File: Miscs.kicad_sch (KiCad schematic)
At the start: 14 parts, among them U7 THGBMUG6C1LBAIL

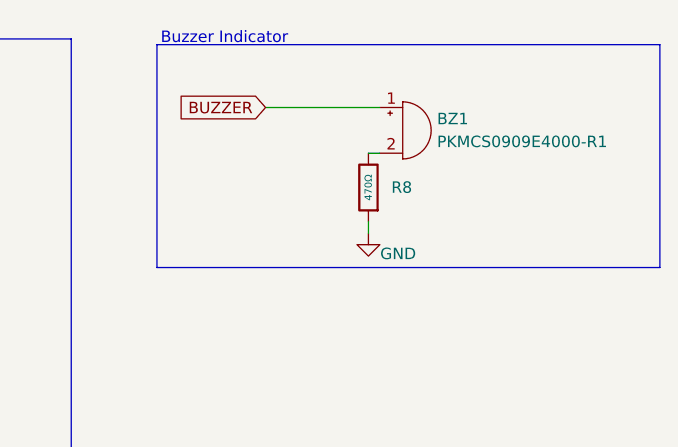
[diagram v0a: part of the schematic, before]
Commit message: Chore: push new design
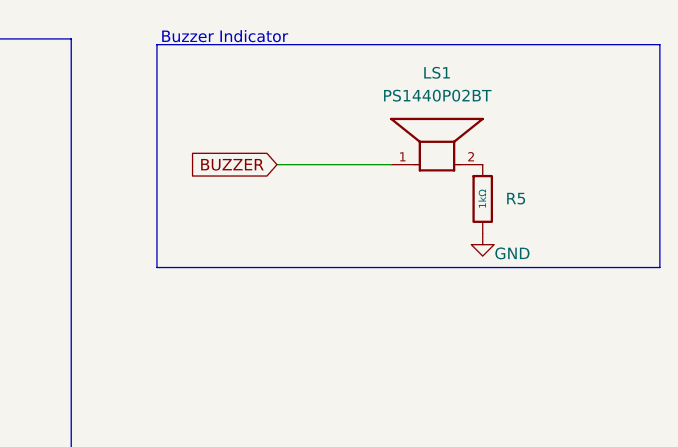
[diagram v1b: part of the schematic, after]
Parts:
- removed BZ1: PKMCS0909E4000-R1, Buzzer_Beeper:PUIAudio_SMT_0825_S_4_R, symbol Device:Buzzer
- removed R8: 470Ω, PCM_JLCPCB:R_0603, symbol PCM_JLCPCB-Resistors:0402,470Ω
- added LS1: PS1440P02BT, Snapeda:PS1440P02BT_BUZZER_PS1440P02BT, symbol Snapeda:PS1440P02BT
- added R5: 1kΩ, PCM_JLCPCB:R_0603, symbol PCM_JLCPCB-Resistors:0603,1kΩ
- C73: footprint PCM_JLCPCB:C_0402 -> PCM_JLCPCB:C_0603
- R49, R50, R51, R52, R53, R54, R55, R56, R57, R58: footprint PCM_JLCPCB:R_0402 -> PCM_JLCPCB:R_0603
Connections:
- net BUZZER: now also LS1.1
- net GND: now also R5.2
- new net: LS1.2, R5.1

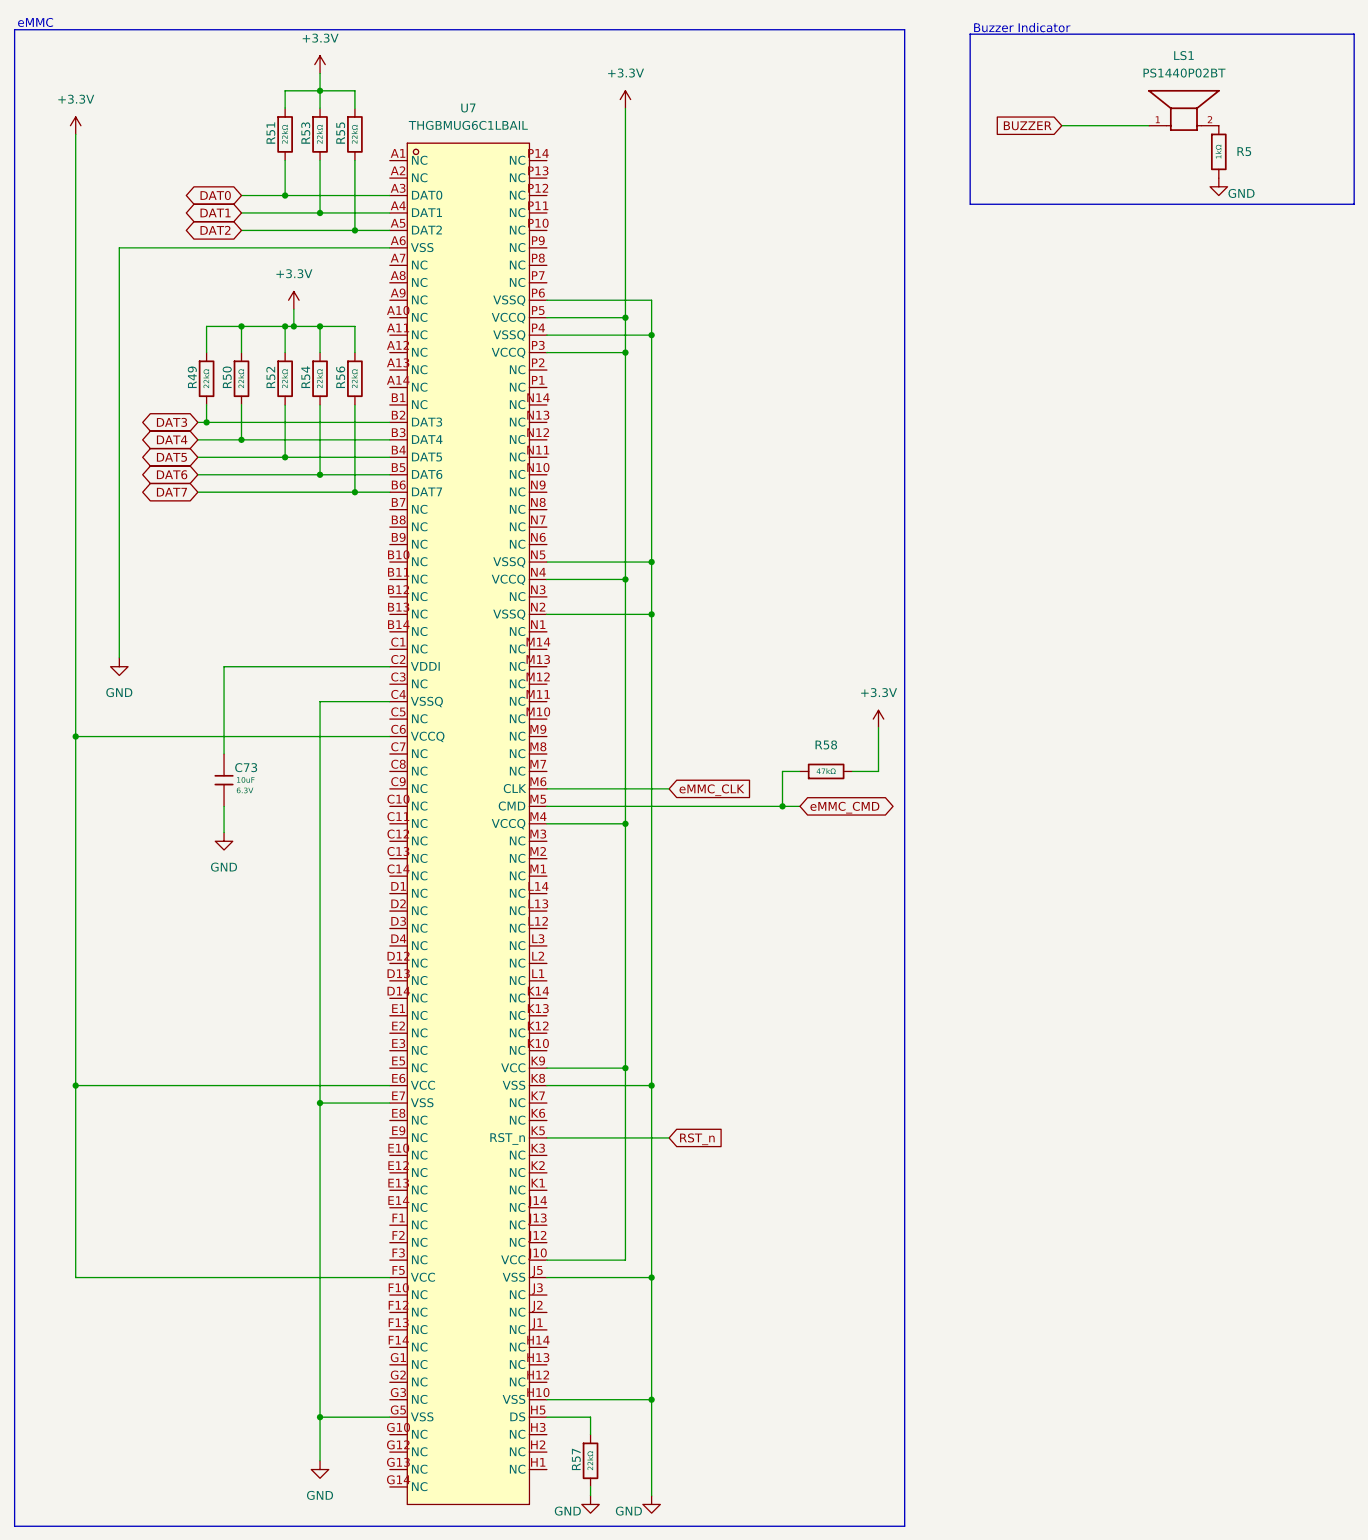
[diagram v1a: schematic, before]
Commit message: Special version
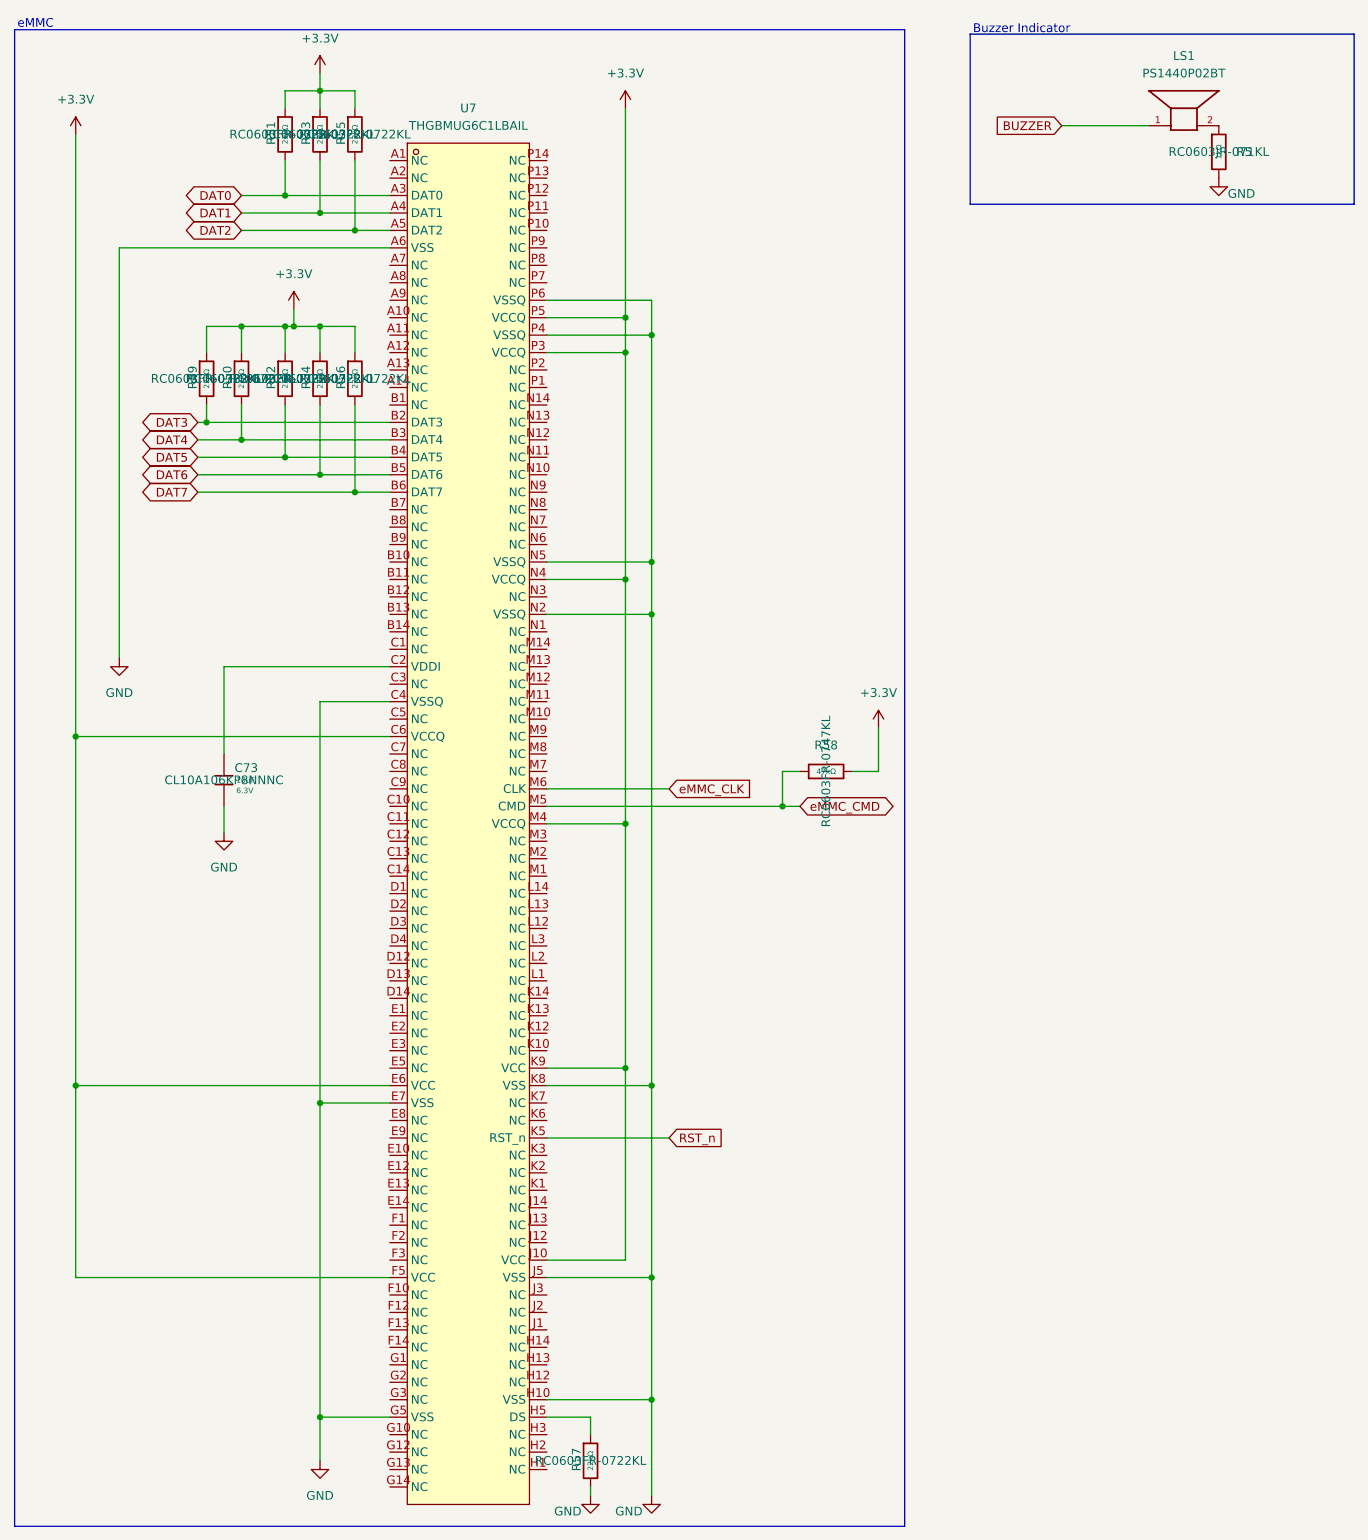
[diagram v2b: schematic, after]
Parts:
- C73: Digikey Parts (none) -> CL10A106KP8NNNC
- R49, R50, R51, R52, R53, R54, R55, R56, R57: Digikey Parts (none) -> RC0603FR-0722KL
- R5: Digikey Parts (none) -> RC0603JR-071KL
- R58: Digikey Parts (none) -> RC0603FR-0747KL
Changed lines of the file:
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@@
 			)
 		)
+		(property "Digikey Parts" "RC0603FR-0722KL"
+			(at 72.39 78.74 0)
+			(effects
+				(font
+					(size 1.27 1.27)
+				)
+			)
+		)
 		(pin "1"
 		)
@@
 			)
 		)
+		(property "Digikey Parts" "CL10A106KP8NNNC"
+			(at 53.34 137.16 0)
+			(effects
+				(font
+					(size 1.27 1.27)
+				)
+			)
+		)
 		(pin "2"
 		)
@@
 			)
 		)
+		(property "Digikey Parts" ""
+			(at 193.04 39.37 0)
+			(effects
+				(font
+					(size 1.27 1.27)
+				)
+			)
+		)
 		(pin "1"
 		)
@@
 			)
 		)
+		(property "Digikey Parts" "RC0603FR-0722KL"
+			(at 67.31 43.18 0)
+			(effects
+				(font
+					(size 1.27 1.27)
+				)
+			)
+		)
 		(pin "1"
 		)
@@
 			)
 		)
+		(property "Digikey Parts" "RC0603FR-0722KL"
+			(at 67.31 78.74 0)
+			(effects
+				(font
+					(size 1.27 1.27)
+				)
+			)
+		)
 		(pin "1"
 		)
@@
 			)
 		)
+		(property "Digikey Parts" "RC0603FR-0722KL"
+			(at 50.8 78.74 0)
+			(effects
+				(font
+					(size 1.27 1.27)
+				)
+			)
+		)
 		(pin "1"
 		)
@@
 			)
 		)
+		(property "Digikey Parts" "RC0603FR-0722KL"
+			(at 62.23 43.18 0)
+			(effects
+				(font
+					(size 1.27 1.27)
+				)
+			)
+		)
 		(pin "1"
 		)
@@
 			)
 		)
+		(property "Digikey Parts" ""
+			(at 90.17 143.51 0)
+			(effects
+				(font
+					(size 1.27 1.27)
+				)
+			)
+		)
 		(pin "A13"
 		)
@@
 			)
 		)
+		(property "Digikey Parts" "RC0603FR-0722KL"
+			(at 72.39 43.18 0)
+			(effects
+				(font
+					(size 1.27 1.27)
+				)
+			)
+		)
 		(pin "1"
 		)
@@
 			)
 		)
+		(property "Digikey Parts" "RC0603JR-071KL"
+			(at 198.12 45.72 0)
+			(effects
+				(font
+					(size 1.27 1.27)
+				)
+			)
+		)
 		(pin "1"
 		)
@@
 			)
 		)
+		(property "Digikey Parts" "RC0603FR-0722KL"
+			(at 55.88 78.74 0)
+			(effects
+				(font
+					(size 1.27 1.27)
+				)
+			)
+		)
 		(pin "1"
 		)
@@
 			)
 		)
+		(property "Digikey Parts" "RC0603FR-0747KL"
+			(at 140.97 135.89 0)
+			(effects
+				(font
+					(size 1.27 1.27)
+				)
+			)
+		)
 		(pin "2"
 		)
@@
 			)
 		)
+		(property "Digikey Parts" "RC0603FR-0722KL"
+			(at 62.23 78.74 0)
+			(effects
+				(font
+					(size 1.27 1.27)
+				)
+			)
+		)
 		(pin "1"
 		)
@@
 			(at 106.68 236.22 0)
 			(effects
+				(font
+					(size 1.27 1.27)
+				)
+			)
+		)
+		(property "Digikey Parts" "RC0603FR-0722KL"
+			(at 106.68 236.22 0)
+			(effects
